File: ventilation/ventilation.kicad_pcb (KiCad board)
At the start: 2 copper layers, 38 x 27 mm, 37 parts, among them J1 Conn_01x03_Pin, J2 Conn_01x04_Pin, J3 Conn_01x04_Pin, J4 Conn_01x04_Pin, J7 Conn_01x02_Pin, Q1 IRLML6402, Q2 BC847, U1 STM32L051C8Tx, U2 MCP1700x-330xxTT

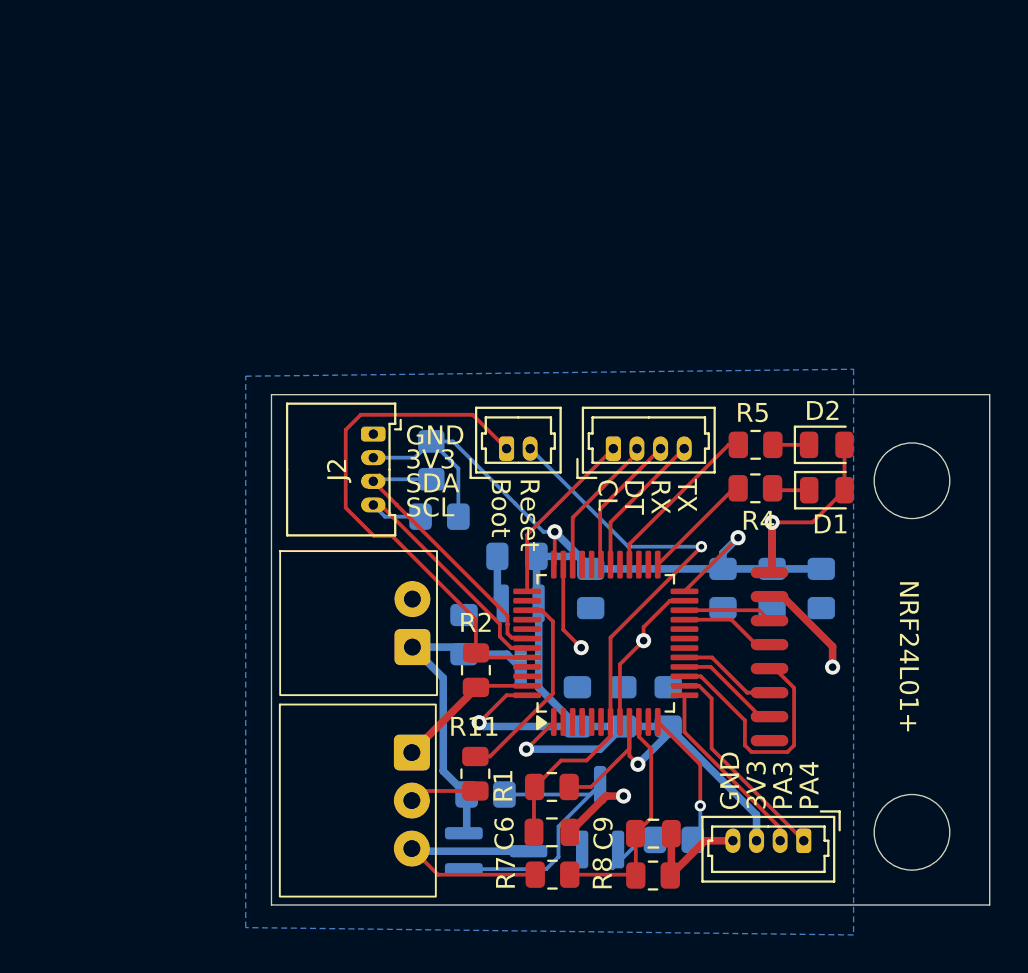
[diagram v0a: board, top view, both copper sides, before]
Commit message: New version
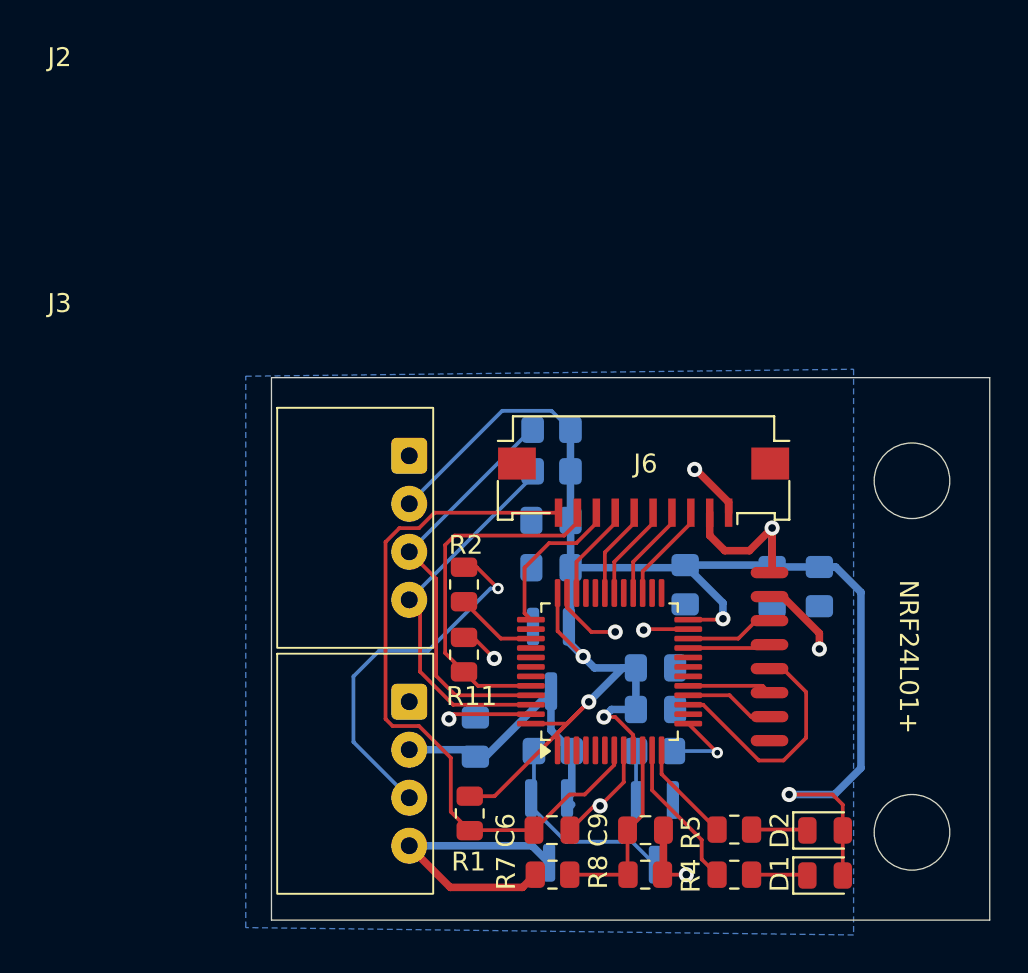
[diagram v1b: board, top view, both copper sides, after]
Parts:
- removed C5: 100n, Capacitor_SMD:C_0805_2012Metric_Pad1.18x1.45mm_HandSolder
- removed J1: Conn_01x03_Pin, PVDW_custom:Connector_1x3_p2.54_hortizontal
- removed J4: Conn_01x04_Pin, PVDW_custom:Molex_PicoBlade_1x04_P1.25mm_Vertical
- removed J5: ~, PVDW_custom:Connector_1x2_p2.54_horizontal
- removed J7: Conn_01x02_Pin, PVDW_custom:Molex_PicoBlade_P1.25mm_Vertical
- added J6: Conn_01x10_Pin, PVDW_custom:FFC_1x10_P1.00mm_Horizontal, F.Cu at (177.2, 80.1)
- J2: footprint PVDW_custom:Molex_PicoBlade_53048-0410_1x04_P1.25mm_Horizontal -> PVDW_custom:Connector_1x4_p2.54_hortizontal
- J3: footprint PVDW_custom:Molex_PicoBlade_1x04_P1.25mm_Vertical -> PVDW_custom:Connector_1x4_p2.54_hortizontal
- moved J3 23.6 mm to (164.8, 98.5)
- moved R4 20.5 mm to (182.0, 100.0)
- moved D2 20.4 mm to (186.8, 97.7)
- moved R5 20.4 mm to (182.0, 97.7)
- moved D1 20.4 mm to (186.8, 100.1)
- moved R11 10.0 mm to (167.7, 84.7), turned to -90 degrees
- moved J2 8.97 mm to (164.8, 85.5), turned to 0 degrees
- moved C4 7.26 mm to (179.4, 84.7), turned to -90 degrees
- moved R9 6.56 mm to (172.3, 76.5), turned to 180 degrees
- moved R10 6.40 mm to (172.3, 78.7)
- moved C10 5.46 mm to (168.3, 92.8)
- moved R6 4.81 mm to (177.8, 93.5)
- moved C3 4.62 mm to (177.8, 89.1), turned to 0 degrees
- moved R1 4.57 mm to (168.0, 96.8), turned to -90 degrees
- moved R3 4.24 mm to (172.4, 93.5), turned to 0 degrees
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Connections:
- J3 pad 1: /SWCLK -> GND
- J3 pad 2: /SWDIO -> +BATT
- J3 pad 3: /USART1_RX -> /SIG_SERVO
- J3 pad 4: /USART1_TX -> /VCC_SERVO
- U1 pad 11: unconnected-(U1-PA1-Pad11) -> /LED_RED
- U1 pad 12: /SW_SERVO -> /LED_GREEN
- U1 pad 13: /PA3 -> /SW_SERVO
- U1 pad 14: /PA4 -> unconnected-(U1-PA4-Pad14)
- U1 pad 25: /LED_RED -> unconnected-(U1-PB12-Pad25)
- U1 pad 27: unconnected-(U1-PB14-Pad27) -> /PB14
- U1 pad 28: /LED_GREEN -> /PB15
- U1 pad 42: /I2C_SCL -> unconnected-(U1-PB6-Pad42)
- U1 pad 43: /I2C_SDA -> unconnected-(U1-PB7-Pad43)
- U1 pad 45: unconnected-(U1-PB8-Pad45) -> /I2C_SCL
- U1 pad 46: unconnected-(U1-PB9-Pad46) -> /I2C_SDA
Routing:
- net /SIG_SERVO: track 3.57 -> 19.5 mm, vias 0 -> 1
- net /PA4: track 11.3 -> 0.00 mm
- net GND: track 39.3 -> 29.4 mm, vias 4 -> 8
- net /PA3: track 9.79 -> 0.00 mm
- net /BOOT: track 27.6 -> 19.0 mm
- net /RESET: track 31.2 -> 38.0 mm, vias 1 -> 0
- net Net-(U1-PB3): track 10.9 -> 4.35 mm
- net /I2C_SCL: track 16.2 -> 21.8 mm
- net /I2C_SDA: track 14.6 -> 20.1 mm
- net /PB14: track 0.00 -> 5.30 mm
- net /PB15: track 0.00 -> 5.10 mm
- net /G_FET: track 15.8 -> 11.0 mm
- net /LED_GREEN: track 9.02 -> 5.41 mm
- net +3V3: track 104.5 -> 107.6 mm
- net /SW_SERVO: track 7.34 -> 4.52 mm
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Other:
- board size 38 x 27 mm -> 38 x 28.7 mm
